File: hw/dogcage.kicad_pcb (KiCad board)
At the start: 2 copper layers, 68.6 x 49.8 mm, 23 parts, among them CON1 BARREL_JACK, P1 Door, P2 Lock, Q1 TIP120, Q2 TIP120, SW1 SW_PUSH, SW2 SW_PUSH, U1 LD1117S50TR, U2 LD1117S33TR, U3 TEENSYLC, U4 ESP-01v090

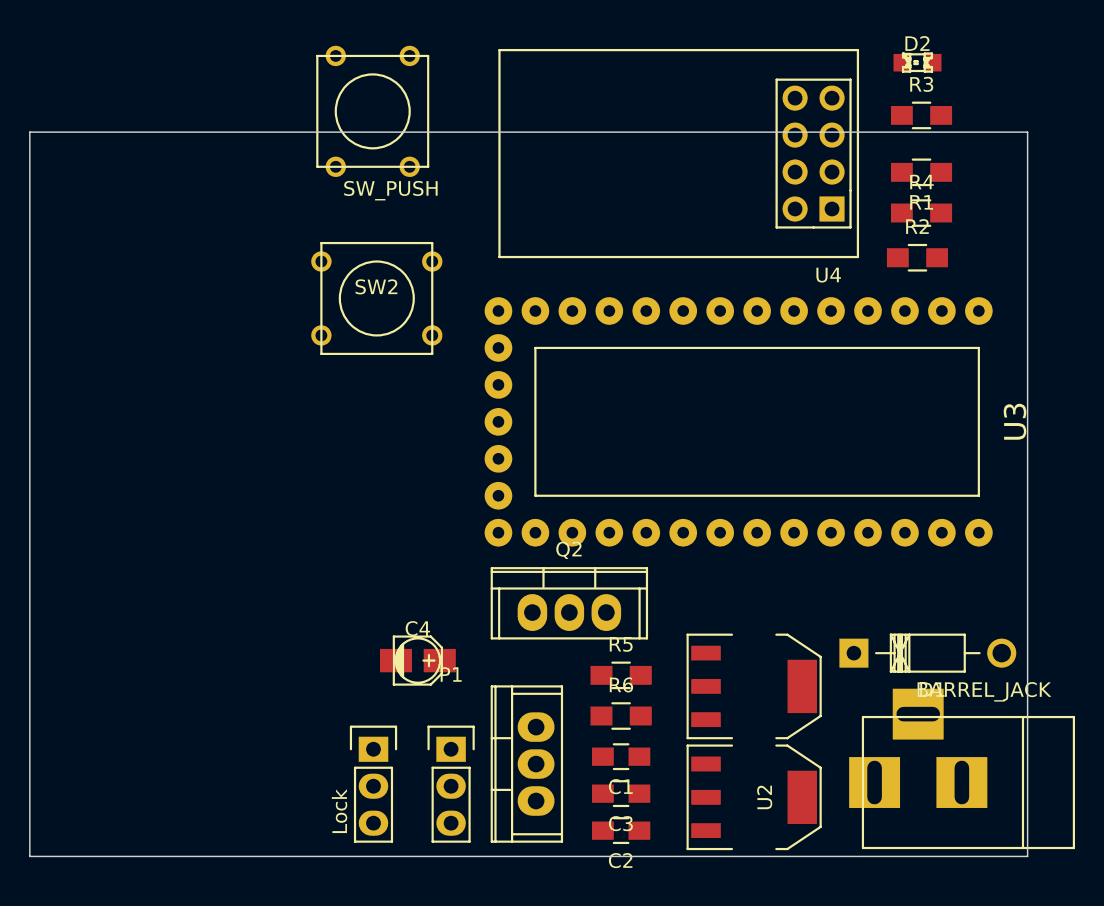
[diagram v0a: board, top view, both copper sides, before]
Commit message: Placement is essentially done
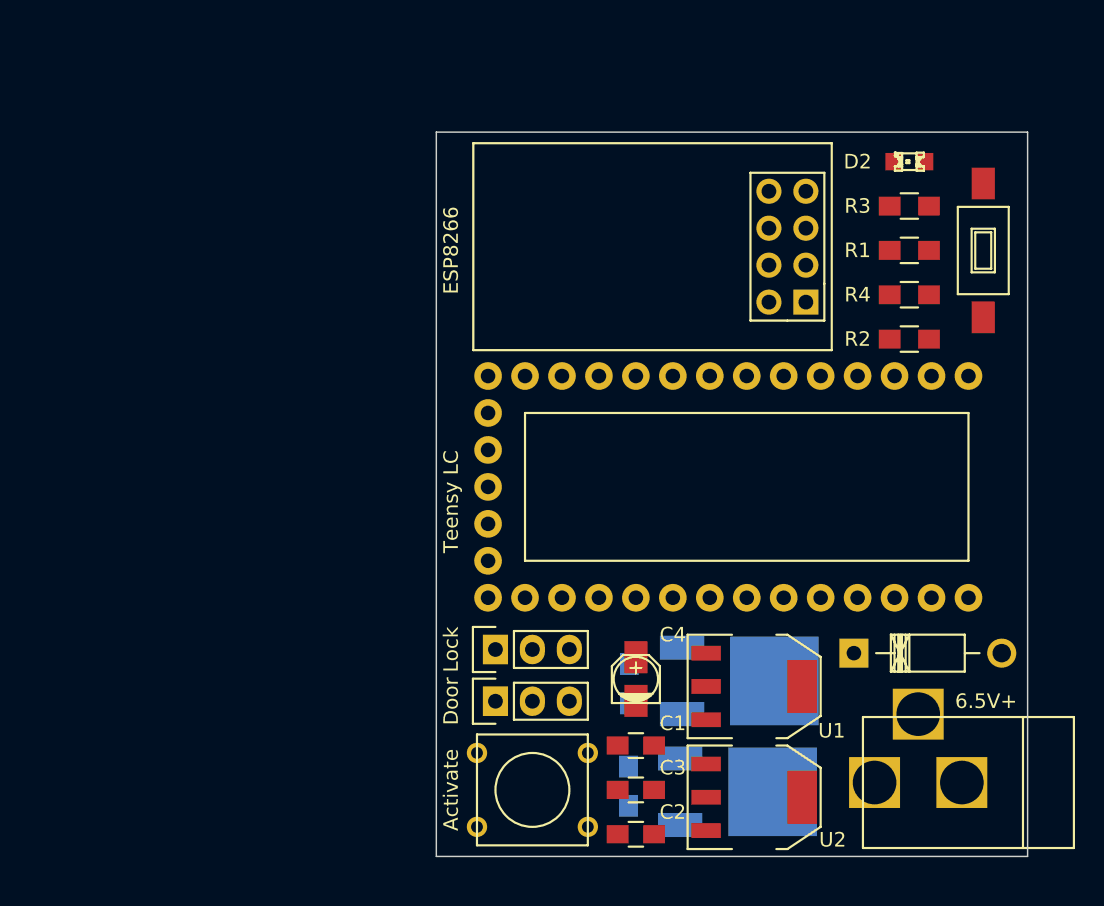
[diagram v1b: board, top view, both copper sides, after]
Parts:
- removed SW1: SW_PUSH, Buttons_Switches_ThroughHole:SW_PUSH_SMALL
- added Activate: SW_PUSH, Buttons_Switches_ThroughHole:SW_PUSH_SMALL, F.Cu at (164.1, 170.7)
- CON1: value BARREL_JACK -> 6.5V+; footprint Connect:BARREL_JACK -> modules:BARREL_JACK-ROUND_TH
- Q1, Q2: value TIP120 -> Darl_NPN; footprint Power_Integrations:TO-220 -> SMD_Packages:DPAK-2; moved to B.Cu
- R5, R6: moved to B.Cu
- SW2: footprint Buttons_Switches_ThroughHole:SW_PUSH_SMALL -> Buttons_Switches_SMD:SW_SPST_FSMSM
- U3: value TEENSYLC -> Teensy LC
- U4: value ESP-01v090 -> ESP8266
- moved SW2 41.8 mm to (195.1, 133.6), turned to 270 degrees
- moved C4 15.0 mm to (171.2, 163.1), turned to 90 degrees
- moved P2 10.8 mm to (161.5, 161.0), turned to 90 degrees
- moved Q1 10.1 mm to (174.2, 170.8)
- moved Q2 9.06 mm to (174.4, 163.2), turned to 90 degrees
- moved D2 6.83 mm to (190.0, 127.5)
- moved U4 6.65 mm to (182.9, 137.2)
- moved R3 6.28 mm to (190.0, 130.6)
- moved R4 5.67 mm to (190.0, 136.7), turned to 180 degrees
- moved R2 5.62 mm to (190.0, 139.7), turned to 180 degrees
- moved R1 5.43 mm to (190.0, 133.6)
- moved R6 4.85 mm to (170.7, 170.4), turned to 90 degrees
- moved U3 4.53 mm to (191.5, 142.2)
- moved P1 4.49 mm to (161.5, 164.6), turned to 90 degrees
- moved C1 1.27 mm to (171.2, 167.6)
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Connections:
- Q1 pad 1: Net-(Q1-Pad1) -> GND
- Q1 pad 2: Net-(P1-Pad3) -> Net-(Q1-Pad2)
- Q1 pad 3: GND -> Net-(P1-Pad3)
- Q2 pad 1: Net-(Q2-Pad1) -> GND
- Q2 pad 2: Net-(P2-Pad3) -> Net-(Q2-Pad2)
- Q2 pad 3: GND -> Net-(P2-Pad3)
- R5 pad 1: /D11 -> /D14
- R5 pad 2: Net-(Q1-Pad1) -> Net-(Q1-Pad2)
- R6 pad 1: /D12 -> /D15
- R6 pad 2: Net-(Q2-Pad1) -> Net-(Q2-Pad2)
- U3 pad 13: /D11 -> (no net)
- U3 pad 14: /D12 -> (no net)
- U3 pad 21: (no net) -> /D14
- U3 pad 22: (no net) -> /D15
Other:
- board size 68.6 x 49.8 mm -> 40.6 x 49.8 mm
- board text added: "Tom Manley tom.manley@gmail.com https://github.com/tpmanley/dogcage Version 2.0"
- board text removed: "https://github.com/tpmanley/dogcage Tom Manley tom.manley@gmail.com"
